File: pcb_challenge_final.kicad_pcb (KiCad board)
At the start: 4 copper layers, 46.6 x 27.8 mm, 164 parts, among them J4 Conn_01x04_Pin, J5 Conn_01x04_Pin, Q15 Q_Dual_NPN_PNP_B1E2B2C2E1C1, Q16 Q_Dual_NPN_PNP_B1E2B2C2E1C1, Q17 Q_Dual_NPN_PNP_B1E2B2C2E1C1, Q18 Q_Dual_NPN_PNP_B1E2B2C2E1C1, Q19 Q_Dual_NPN_PNP_B1E2B2C2E1C1, Q20 Q_Dual_NPN_PNP_B1E2B2C2E1C1, Q21 Q_Dual_NPN_PNP_B1E2B2C2E1C1, Q22 Q_Dual_NPN_PNP_B1E2B2C2E1C1, Q23 Q_Dual_NPN_PNP_B1E2B2C2E1C1, Q24 Q_Dual_NPN_PNP_B1E2B2C2E1C1, Q25 Q_Dual_NPN_PNP_B1E2B2C2E1C1, Q26 Q_Dual_NPN_PNP_B1E2B2C2E1C1, Q27 Q_Dual_NPN_PNP_B1E2B2C2E1C1, Q28 Q_Dual_NPN_PNP_B1E2B2C2E1C1, Q29 Q_Dual_NPN_PNP_B1E2B2C2E1C1, SW1 SW_Push, SW2 SW_MEC_5G, SW3 SW_Push, U1 74AUP1G80, U10 NMUX1308BQ, U11 NMUX1308BQ, U12 NMUX1308BQ, U13 NMUX1308BQ, U14 NMUX1308BQ, U15 NMUX1308BQ, U16 NMUX1308BQ, U17 74AUP1G80, U18 74AHC1G86, U19 74AUP1G80, U20 74AUP1G80, U21 74LV1T08GV, U22 CD74HC283M96, U23 74LV1T08GV, U24 74LVC1GU04DRL, U25 ESP32-S3-MINI-1, U26 74LVC1GU04DRL, U27 74LV1T08GV, U28 CD74HC283M96, U29 NMUX1308BQ, U3 74AHC1G86, U30 NMUX1308BQ, U31 NMUX1308BQ, U32 NMUX1308BQ, U33 74AUP1G80, U34 74AUP1G80, U35 NMUX1308BQ, U36 NMUX1308BQ, U37 74AUP1G80, U38 74AUP1G80, U39 NMUX1308BQ, U4 74AUP1G80, U40 NMUX1308BQ, U41 NMUX1308BQ, U42 NMUX1308BQ, U43 NMUX1308BQ, U44 NMUX1308BQ, U45 74AUP1G80, U46 74AUP1G80, U47 74AUP1G80, U48 74AUP1G80, U49 74AUP1G80, U5 74AUP1G80, U50 74AUP1G80, U51 74LV1T08GV, U52 74AHC1G86, U53 74LVC1GU04DRL, U54 74LVC1GU04DRL, U55 74AHC1G86, U56 74AHC1G86, U57 74LVC1GU04DRL, U58 74LVC1GU04DRL, U59 74LV1T08GV, U6 74AUP1G80, U60 74AHC1G86, U61 74LVC1GU04DRL, U62 74LV1T08GV, U63 74LV1T08GV, U64 NMUX1308BQ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

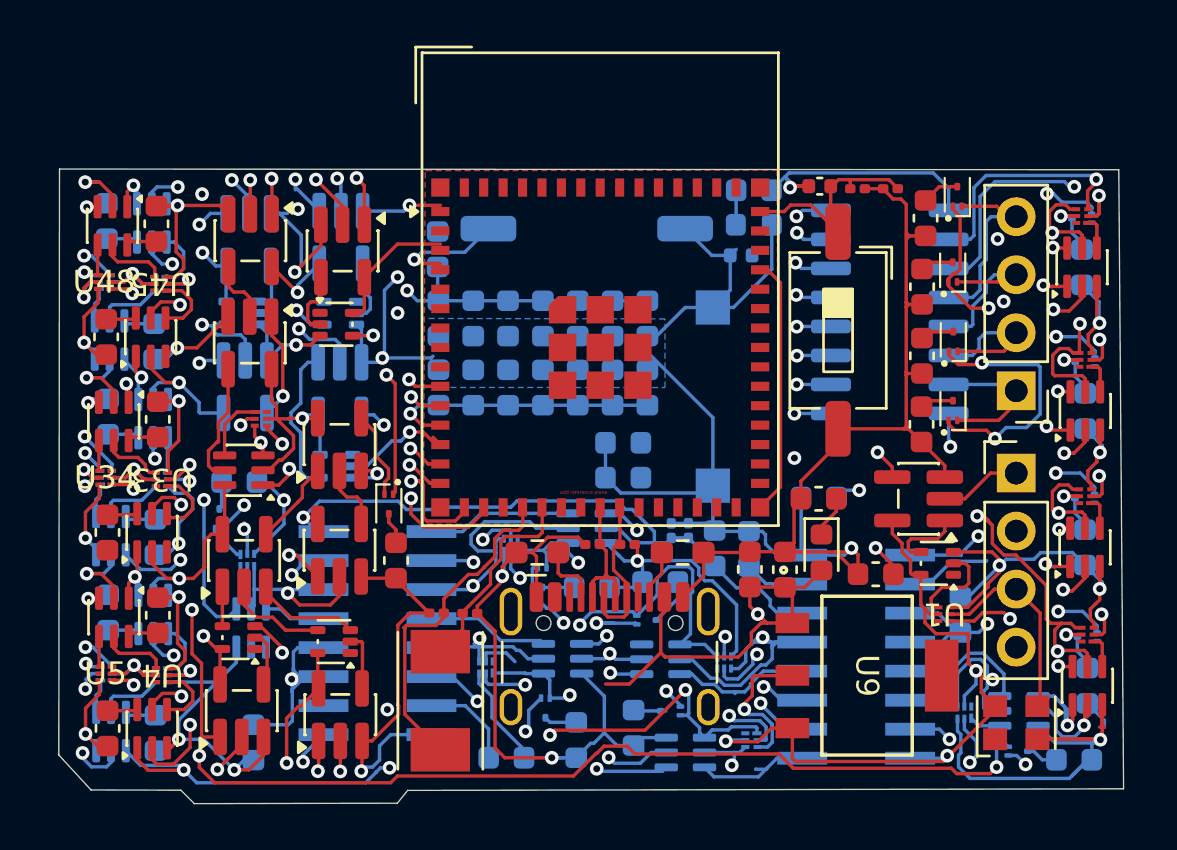
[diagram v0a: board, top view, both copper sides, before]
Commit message: Add files via upload
fixed the connections
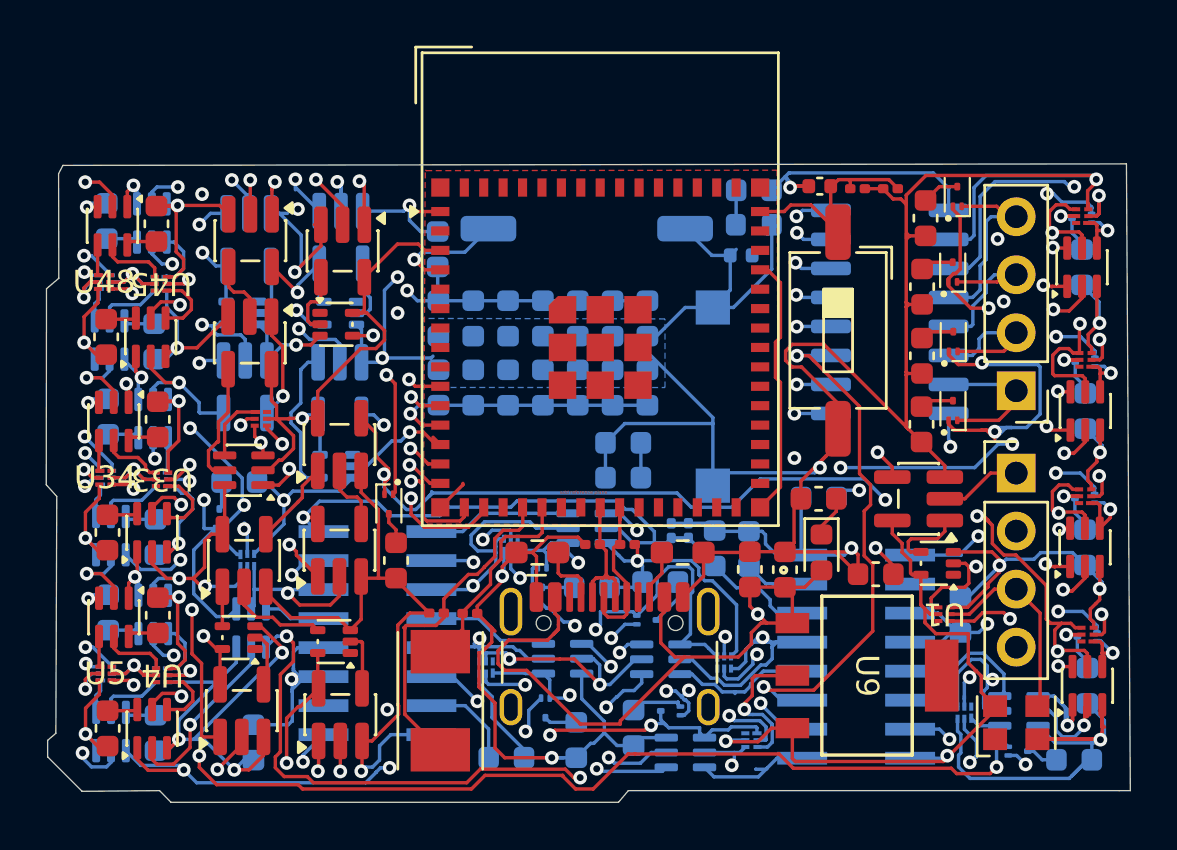
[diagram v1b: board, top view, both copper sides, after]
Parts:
- renumbered R to R28
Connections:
- Q19 pad 1: IO8 -> Net-(Q19A-B1)
- Q19 pad 2: rw2 -> IO8
- Q19 pad 3: Net-(Q19A-E1) -> rw2
- R38 pad 2: Net-(Q19A-E1) -> Net-(Q19A-B1)
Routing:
- net GND: track 439.4 -> 504.0 mm, vias 37 -> 38
- net wr2: track 5.79 -> 69.4 mm
- net IO12: track 8.88 -> 41.1 mm, vias 2 -> 4
- net R_en: track 30.5 -> 60.9 mm, vias 4 -> 6
- net rw1: track 13.8 -> 39.8 mm
- net +3.3V: track 338.3 -> 364.1 mm, vias 34 -> 36
- net Net-(Q16A-C1): track 18.2 -> 43.1 mm, vias 1 -> 3
- net rc2: track 43.8 -> 63.7 mm
- net +5V: track 29.6 -> 42.3 mm
- net clk: track 127.4 -> 136.4 mm
- net Net-(U22-A3): track 33.3 -> 24.5 mm
- net rst: track 141.8 -> 150.1 mm, vias 12 -> 13
- net out_1: track 21.3 -> 14.3 mm
- net ???: track 4.05 -> 8.63 mm, vias 0 -> 1
- net rs3: track 3.78 -> 0.81 mm
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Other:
- board size 46.6 x 27.8 mm -> 47.5 x 27.9 mm
